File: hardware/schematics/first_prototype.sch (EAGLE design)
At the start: 11 parts, among them Q1 BSS138, U1 CD74HCT4053M

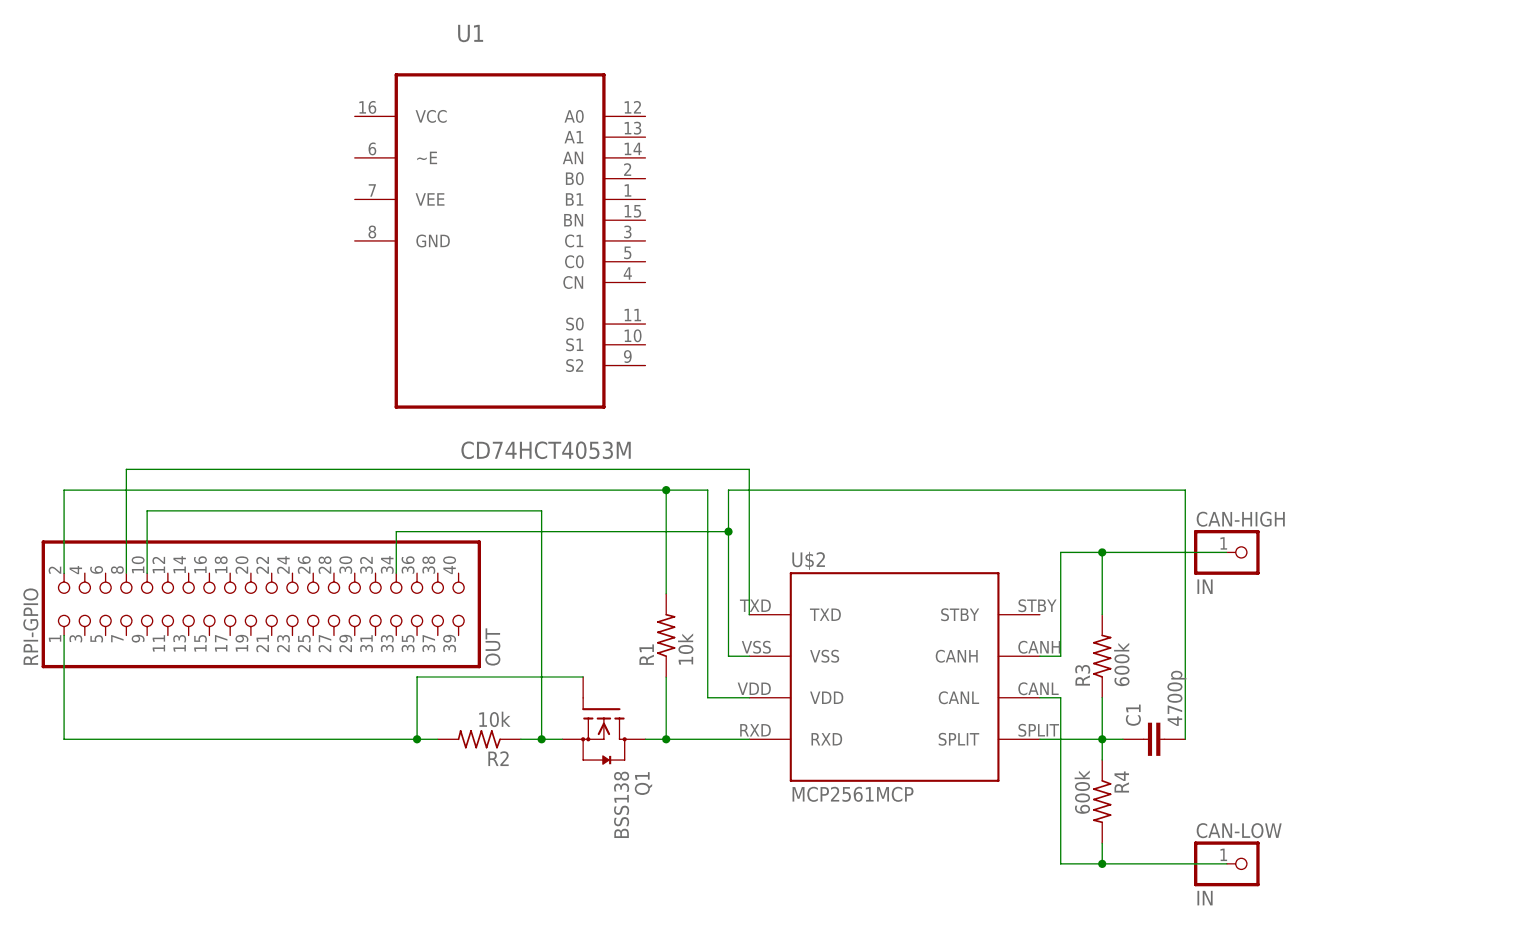
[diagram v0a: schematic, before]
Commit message: pushing changes to schematics
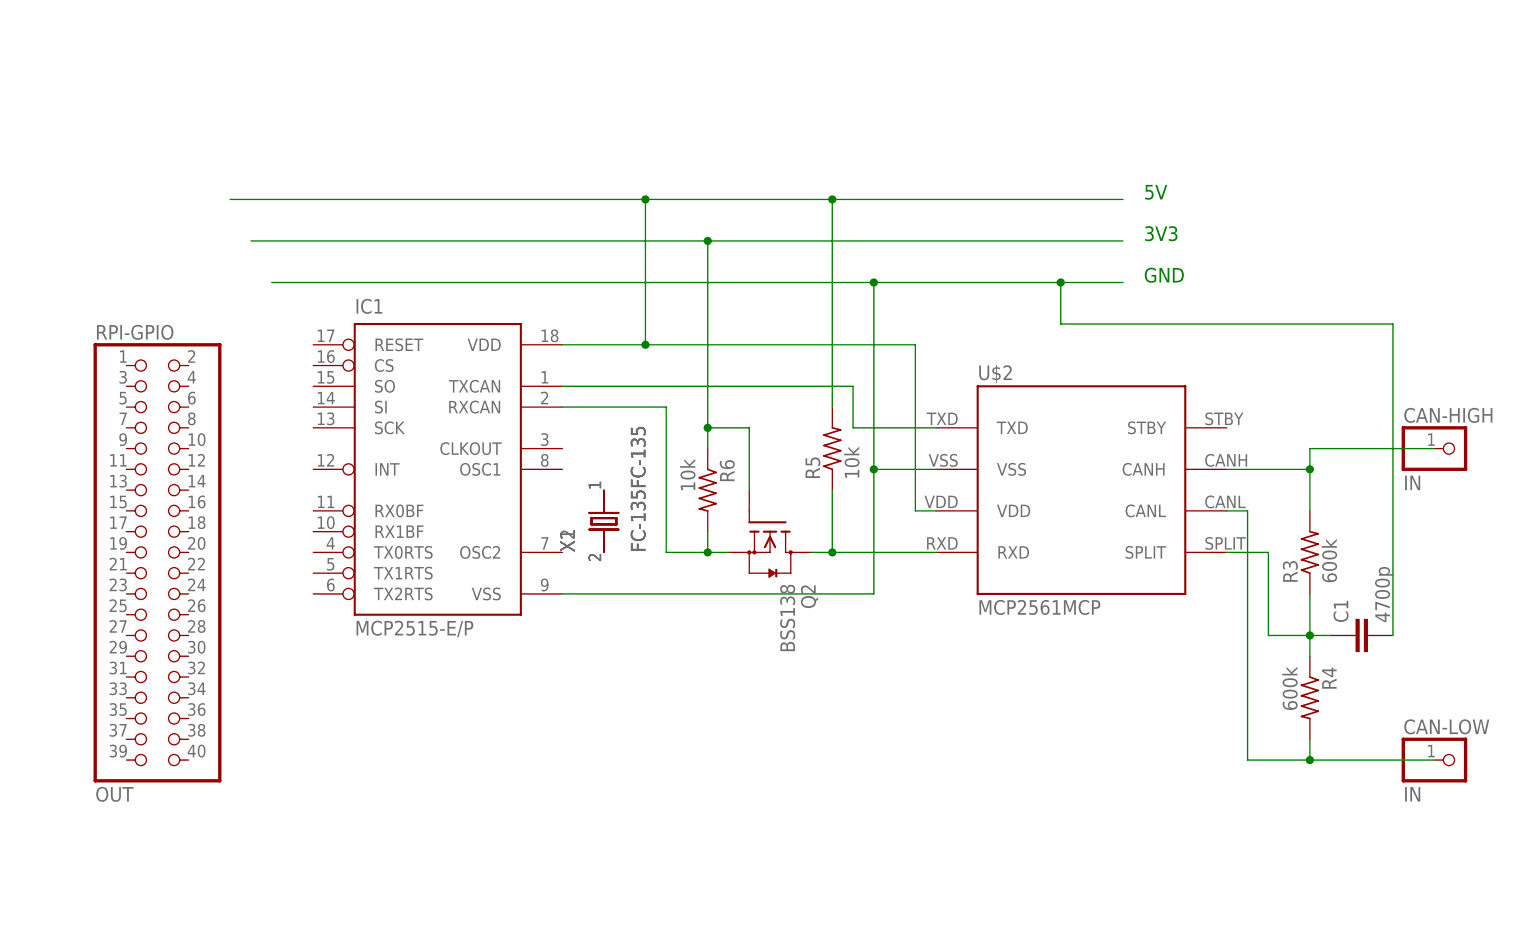
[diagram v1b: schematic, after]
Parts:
- removed Q1: BSS138, m-pad-2.1:BSS138
- removed R1, R2: 10k, rcl:R-US_M2309
- removed U1: CD74HCT4053M, Texas Instruments_By_element14_Batch_1:CD74HCT4053M
- added IC1: MCP2515-E/P, mcp2515:MCP2515-E/P
- added Q2: BSS138, m-pad-2.1:BSS138
- added R5, R6: 10k, rcl:R-US_M2309
- added X1, X2: FC-135FC-135, m-pad-2.1:FC-135FC-135
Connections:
- removed net N$1: Q1.S, R2.1, RPI-GPIO.10
- removed net N$2: Q1.D, R1.1, U$2.RXD
- removed net N$4: R1.2, RPI-GPIO.2, U$2.VDD
- removed net N$6: Q1.G, R2.2, RPI-GPIO.1
- new net N$10: IC1.RXCAN, Q2.S, R6.2
- new net N$11: Q2.D, R5.1, U$2.RXD
- new net N$12: X1.2, X2.2
- new net N$13: X1.1, X2.1
- new net N$15: IC1.VDD, R5.2, U$2.VDD
- new net N$16: IC1.TXCAN, U$2.TXD
- net N$3: now also Q2.G, R6.1; no longer RPI-GPIO.8, U$2.TXD
- net N$5: now also IC1.VSS; no longer RPI-GPIO.34
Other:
- note added: "3V3"
- note added: "5V"
- note added: "GND"
- moved on the sheet: C1, CAN-HIGH, CAN-LOW, R3, R4, RPI-GPIO, U$2
